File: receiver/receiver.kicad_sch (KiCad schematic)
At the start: 0 parts

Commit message: devlog 02
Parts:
- added C1: 100nF, symbol Device:C
- added C2: 10uF, symbol Device:C
- added C3: 1uF, symbol Device:C
- added D_ACT: ACT, symbol Device:LED
- added HDR1: DEBUG, symbol Connector_Generic:Conn_01x03
- added J1: USB-C, symbol Connector:USB_C_Receptacle_USB2.0_16P
- added R_ACT: 1k, symbol Device:R
- added R_CC1, R_CC2: 5.1k, symbol Device:R
- added R_EN: 10k, symbol Device:R
- added SW_BOOT: BOOT, symbol Switch:SW_Push
- added SW_RST: RESET, symbol Switch:SW_Push
- added U1: ESP32-S3-WROOM-1, symbol RF_Module:ESP32-S3-WROOM-1
- added U2: AP2112K-3.3, symbol Regulator_Linear:AP2112K-3.3
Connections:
- new net: J1.A1 (GND), J1.A12 (GND), J1.B1 (GND), J1.B12 (GND)
- new net: J1.A4 (VBUS), J1.A9 (VBUS), J1.B4 (VBUS), J1.B9 (VBUS)
- new net: U1.1 (GND), U1.40 (GND), U1.41 (GND)
- no-connect marks 0 -> 2

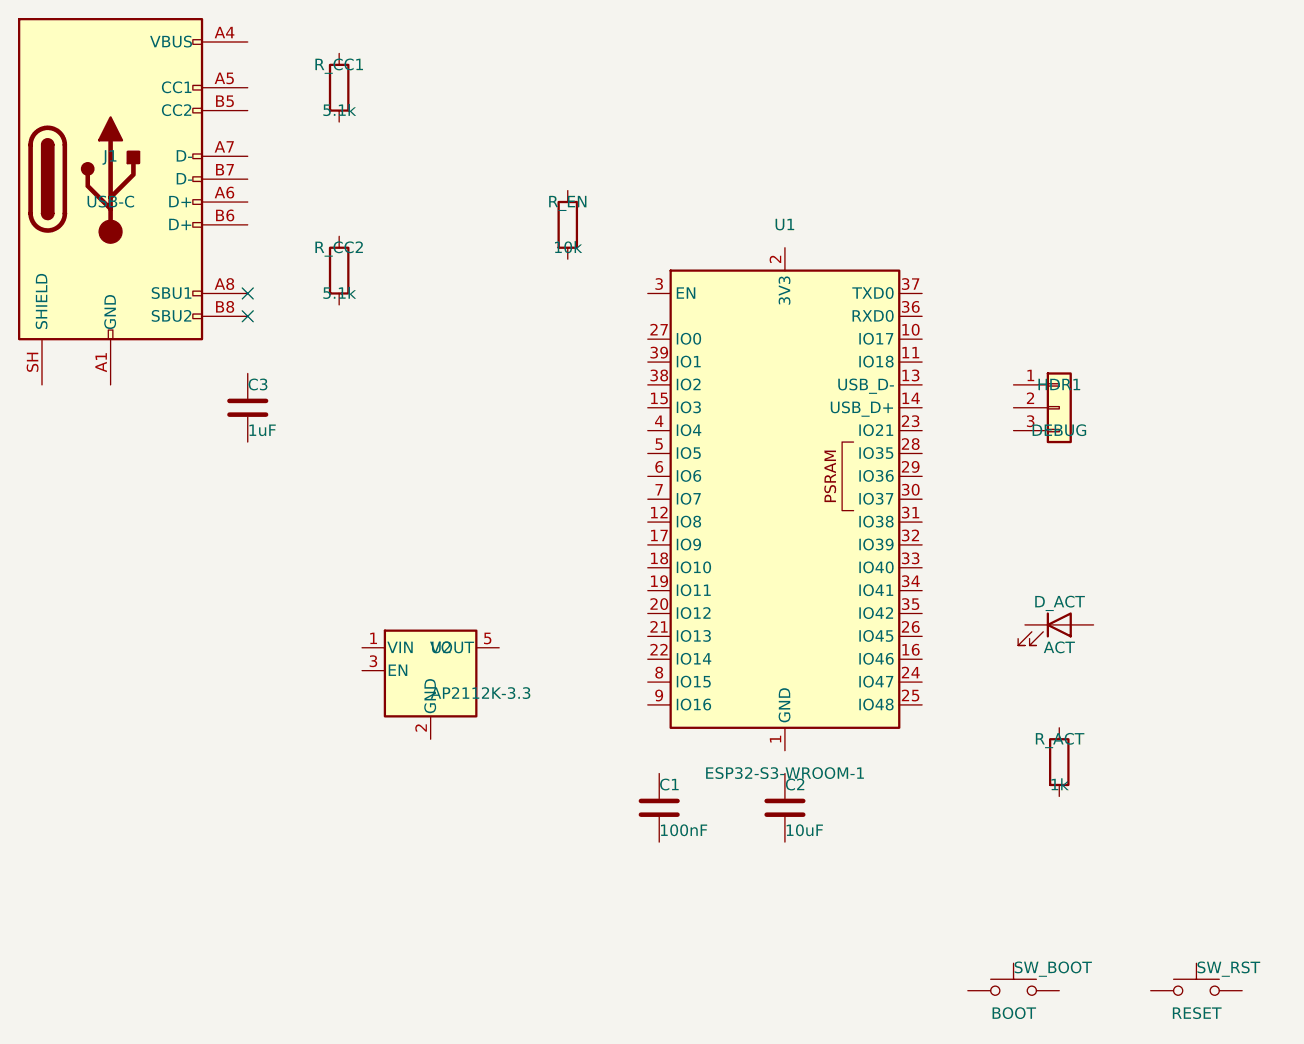
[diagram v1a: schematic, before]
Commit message: devlog 03
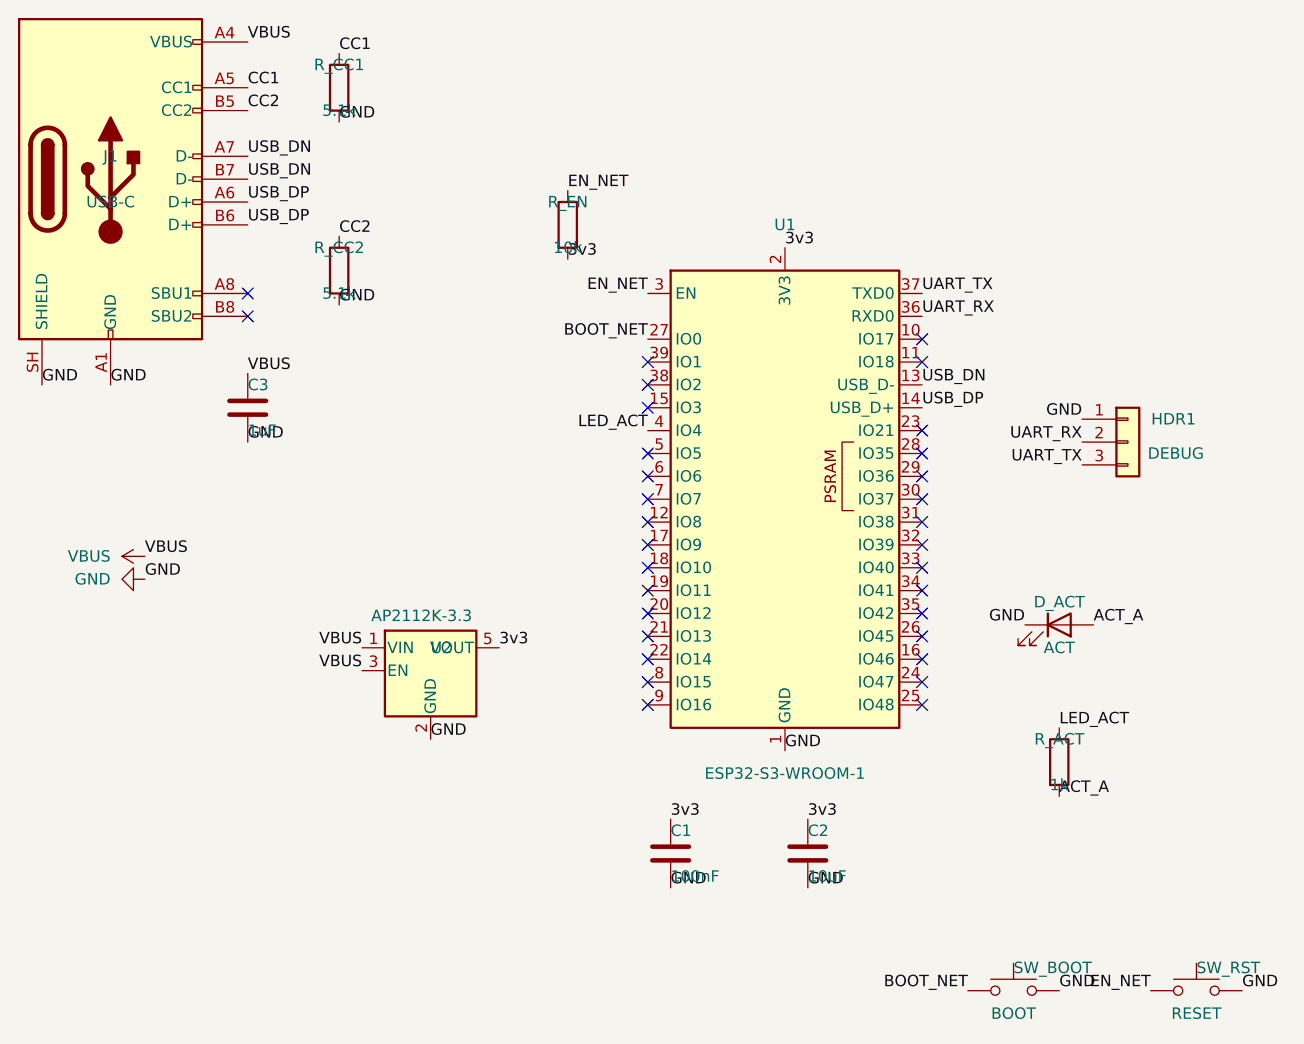
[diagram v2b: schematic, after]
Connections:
- net 3v3: now reaches C2.1
- net 3v3: now also C1.1, R_EN.2, U1.2 (3V3), U2.5 (VOUT)
- net GND: now reaches C2.2
- net GND: now also C1.2, C3.2, D_ACT.1 (K), HDR1.1 (Pin_1), J1.A1 (GND), J1.A12 (GND), J1.B1 (GND), J1.B12 (GND), J1.SH (SHIELD), R_CC1.2, R_CC2.2, SW_BOOT.2, SW_RST.2, U1.1 (GND), U1.40 (GND), U1.41 (GND), U2.2 (GND)
- net CC2: now reaches R_CC2.1
- net CC2: now also J1.B5 (CC2)
- net UART_RX: now reaches HDR1.2 (Pin_2)
- net UART_RX: now also U1.36 (RXD0)
- net UART_TX: now reaches HDR1.3 (Pin_3)
- net UART_TX: now also U1.37 (TXD0)
- net EN_NET: now reaches R_EN.1
- net EN_NET: now also SW_RST.1, U1.3 (EN)
- net VBUS: now reaches U2.1 (VIN)
- net VBUS: now also C3.1, J1.A4 (VBUS), J1.A9 (VBUS), J1.B4 (VBUS), J1.B9 (VBUS), U2.3 (EN)
- net LED_ACT: now reaches R_ACT.1
- net LED_ACT: now also U1.4 (IO4)
- net ACT_A: now reaches R_ACT.2
- net ACT_A: now also D_ACT.2 (A)
- net CC1: now reaches R_CC1.1
- net CC1: now also J1.A5 (CC1)
- net BOOT_NET: now reaches SW_BOOT.1
- net BOOT_NET: now also U1.27 (IO0)
- net USB_DP: now reaches J1.A6 (D+)
- net USB_DP: now also J1.B6 (D+), U1.14 (USB_D+)
- net USB_DN: now reaches J1.A7 (D-)
- net USB_DN: now also J1.B7 (D-), U1.13 (USB_D-)
- no-connect marks 2 -> 32
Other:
- moved on the sheet: C1, C2, HDR1
